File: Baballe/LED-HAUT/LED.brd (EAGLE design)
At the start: 30 x 32 mm, 15 parts, among them Q1 200mA/50V, Q2 200mA/50V, Q3 200mA/50V

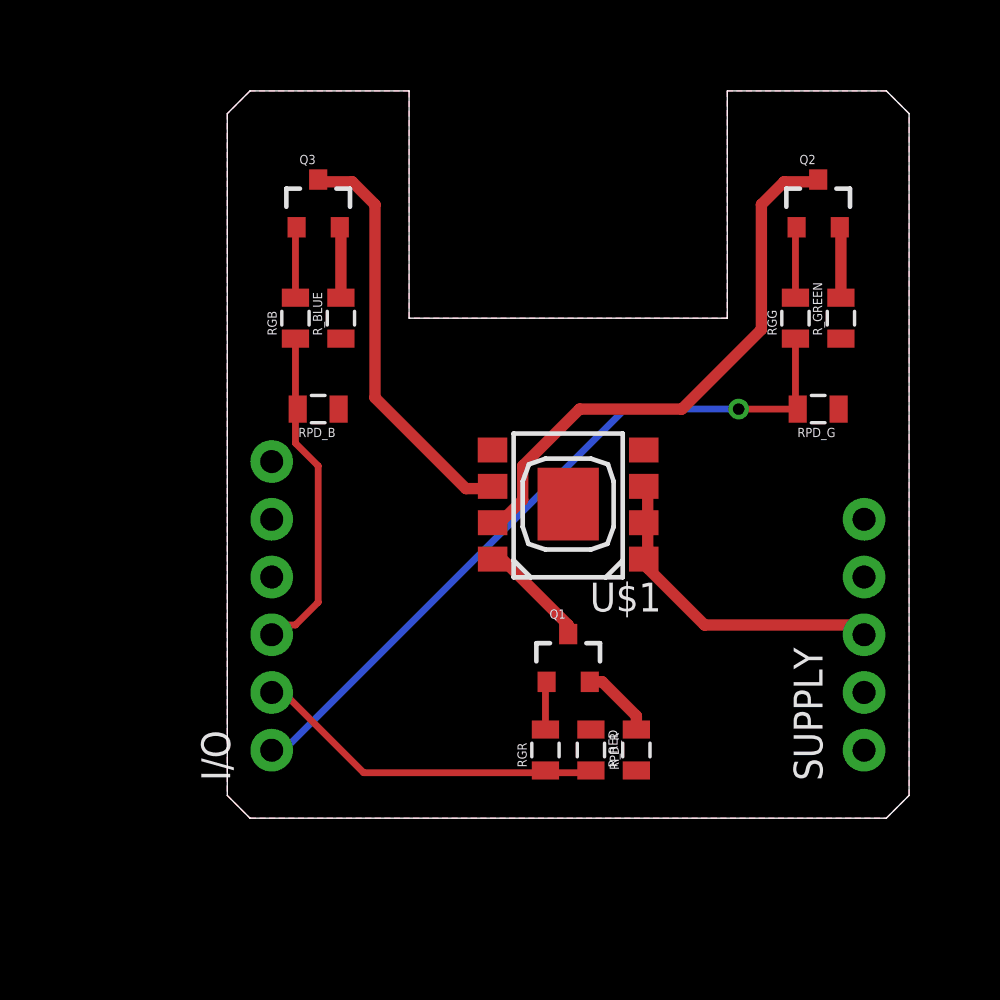
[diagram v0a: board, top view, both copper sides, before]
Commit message: V2 de la Baballe
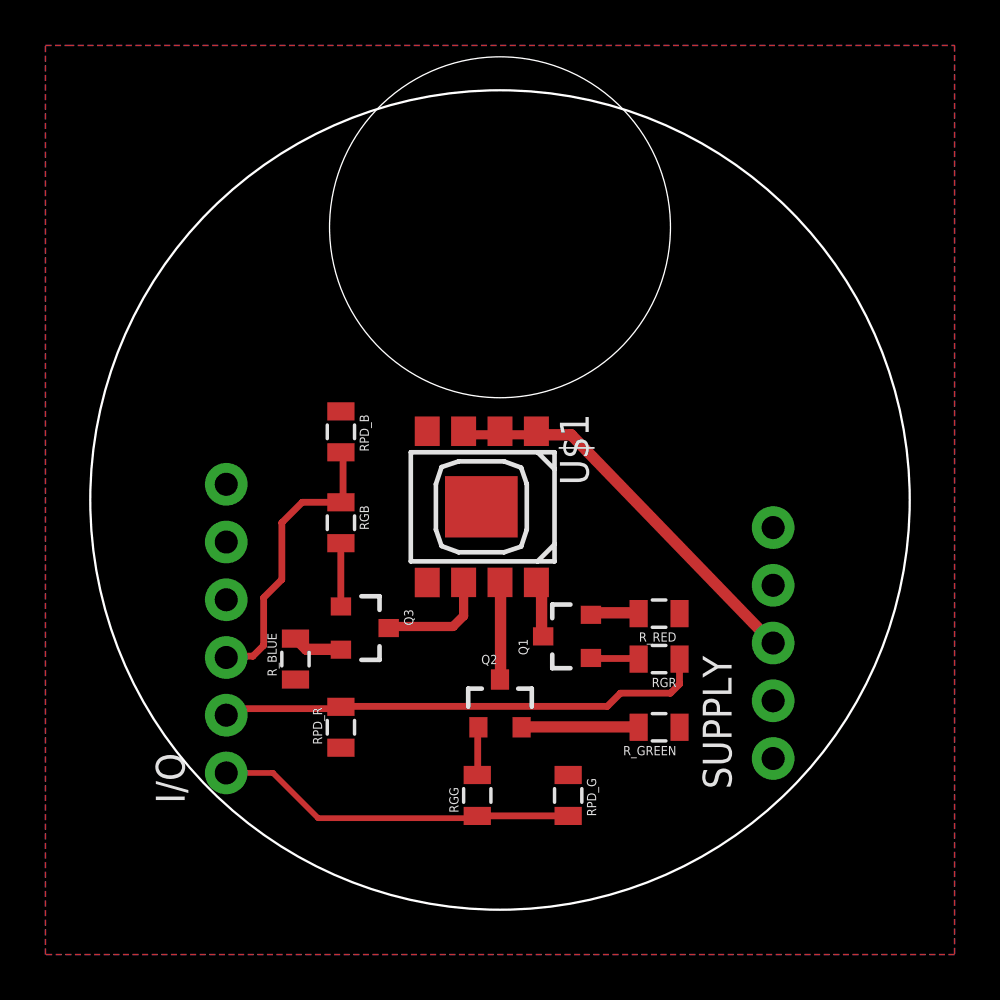
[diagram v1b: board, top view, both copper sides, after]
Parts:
- moved Q2 26.1 mm to (56.0, 5.00)
- moved RGG 25.2 mm to (55.0, 1.00)
- moved RPD_G 20.2 mm to (59.0, 1.00), turned to 270 degrees
- moved R_GREEN 19.7 mm to (63.0, 4.00), turned to 180 degrees
- moved Q3 18.7 mm to (50.0, 8.37), turned to 270 degrees
- moved R_BLUE 15.1 mm to (47.0, 7.00)
- moved RPD_R 11.0 mm to (49.0, 4.00), turned to 90 degrees
- moved RGB 9.22 mm to (49.0, 13.0), turned to 270 degrees
- moved RGR 6.40 mm to (63.0, 7.00), turned to 180 degrees
- moved R_RED 6.08 mm to (63.0, 9.00), turned to 180 degrees
- moved SUPPLY 4.02 mm to (68.0, 2.63)
- moved U$1 3.08 mm to (56.0, 13.7), turned to 270 degrees
- moved I/O 2.24 mm to (44.0, 1.99)
- moved RPD_B 1.41 mm to (49.0, 17.0), turned to 270 degrees
- moved Q1 1.00 mm to (59.0, 8.00), turned to 90 degrees
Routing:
- net N$8: track 24.7 -> 4.82 mm
- net O_GREEN: track 33.1 -> 15.9 mm, vias 1 -> 0
- net N$9: track 18.4 -> 5.51 mm
- net O_RED: track 16.3 -> 21.7 mm
- net V_IN: track 15.0 -> 18.1 mm
- net N$2: track 3.15 -> 5.15 mm
- net N$7: track 4.98 -> 3.04 mm
- net O_BLUE: track 15.0 -> 13.1 mm
- net N$3: track 3.27 -> 2.17 mm
- net N$4: track 3.15 -> 2.12 mm
- net N$1: track 3.15 -> 2.20 mm
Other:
- board size 30 x 32 mm -> 36.1 x 36.1 mm
